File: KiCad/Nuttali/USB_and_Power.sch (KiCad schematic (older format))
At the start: 1 part

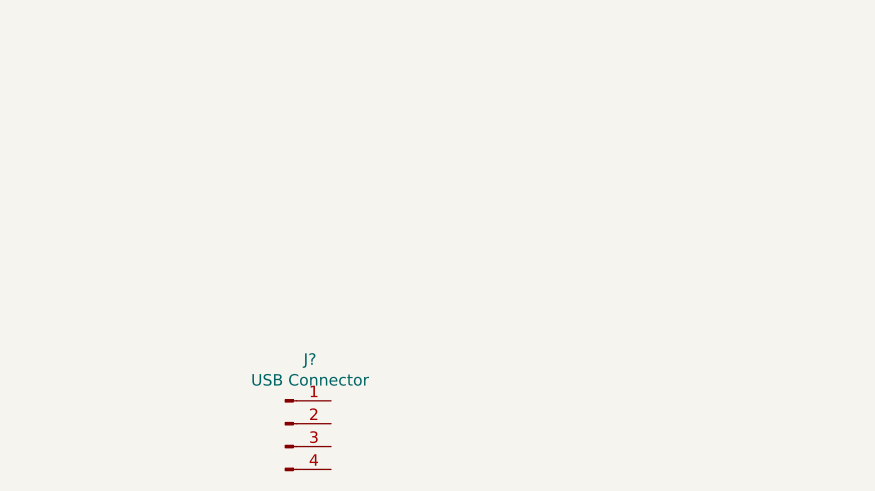
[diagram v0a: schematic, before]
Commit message: Fixed power and USB
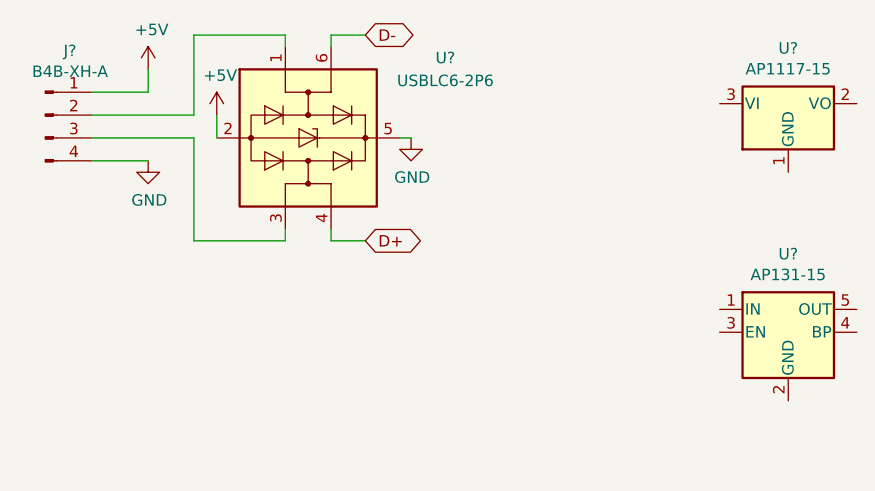
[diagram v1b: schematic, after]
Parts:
- added U?: USBLC6-2P6, Package_TO_SOT_SMD:SOT-666, symbol Power_Protection:USBLC6-2P6
- added U?: AP1117-15, Package_TO_SOT_SMD:SOT-223-3_TabPin2, symbol Regulator_Linear:AP1117-15
- added U?: AP131-15, Package_TO_SOT_SMD:SOT-23-5, symbol Regulator_Linear:AP131-15
- J?: value USB Connector -> B4B-XH-A
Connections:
- net +5V: now reaches J?.1 (Pin_1)
- net +5V: now also U?.2 (GND)
- net at J?.2 (Pin_2): now also U?.1 (I/O1)
- net at J?.3 (Pin_3): now also U?.3 (I/O2)
- net GND: now reaches J?.4 (Pin_4)
- net GND: now also U?.5 (VBUS)
- new net D+: U?.4 (I/O2)
- new net D-: U?.6 (I/O1)
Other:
- moved on the sheet: J?
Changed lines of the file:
@@
 L Connector:Conn_01x04_Male J?
 U 1 1 601D53F8
-P 2450 3050
-F 0 "J?" H 2558 3331 50  0000 C CNN
-F 1 "USB Connector" H 2558 3240 50  0000 C CNN
-F 2 "" H 2450 3050 50  0001 C CNN
-F 3 "~" H 2450 3050 50  0001 C CNN
-	1    2450 3050
+P 1400 1700
+AR Path="/601D53F8" Ref="J?"  Part="1"
+AR Path="/601D470C/601D53F8" Ref="J?"  Part="1"
+F 0 "J?" H 1508 1981 50  0000 C CNN
+F 1 "B4B-XH-A" H 1508 1890 50  0000 C CNN
+F 2 "" H 1400 1700 50  0001 C CNN
+F 3 "~" H 1400 1700 50  0001 C CNN
+	1    1400 1700
 	1    0    0    -1
 $EndComp
+$Comp
+L power:+5V #PWR?
+U 1 1 6025442C
+P 1850 1500
+F 0 "#PWR?" H 1850 1350 50  0001 C CNN
+F 1 "+5V" H 1865 1673 50  0000 C CNN
+F 2 "" H 1850 1500 50  0001 C CNN
+F 3 "" H 1850 1500 50  0001 C CNN
+	1    1850 1500
+	1    0    0    -1
+$EndComp
+Wire Wire Line
+	1600 1600 1850 1600
+Wire Wire Line
+	1850 1600 1850 1500
+$Comp
+L Power_Protection:USBLC6-2P6 U?
+U 1 1 60257671
+P 2550 1800
+F 0 "U?" V 2200 2400 50  0000 C CNN
+F 1 "USBLC6-2P6" V 2300 2400 50  0000 C CNN
+F 2 "Package_TO_SOT_SMD:SOT-666" H 2550 1300 50  0001 C CNN
+F 3 "https://www.st.com/resource/en/datasheet/usblc6-2.pdf" H 2750 2150 50  0001 C CNN
+	1    2550 1800
+	0    1    1    0
+$EndComp
+Wire Wire Line
+	1600 1700 2050 1700
+Wire Wire Line
+	2050 1700 2050 1350
+Wire Wire Line
+	2050 1350 2450 1350
+Wire Wire Line
+	2450 1350 2450 1400
+Wire Wire Line
+	1600 1800 2050 1800
+Wire Wire Line
+	2050 1800 2050 2250
+Wire Wire Line
+	2050 2250 2450 2250
+Wire Wire Line
+	2450 2250 2450 2200
+$Comp
+L power:+5V #PWR?
+U 1 1 60263555
+P 2150 1700
+F 0 "#PWR?" H 2150 1550 50  0001 C CNN
+F 1 "+5V" H 2165 1873 50  0000 C CNN
+F 2 "" H 2150 1700 50  0001 C CNN
+F 3 "" H 2150 1700 50  0001 C CNN
+	1    2150 1700
+	1    0    0    -1
+$EndComp
+Wire Wire Line
+	2150 1800 2150 1700
+Wire Wire Line
+	1600 1900 1850 1900
+$Comp
+L power:GND #PWR?
+U 1 1 60263C21
+P 1850 1900
+F 0 "#PWR?" H 1850 1650 50  0001 C CNN
+F 1 "GND" H 1855 1727 50  0000 C CNN
+F 2 "" H 1850 1900 50  0001 C CNN
+F 3 "" H 1850 1900 50  0001 C CNN
+	1    1850 1900
+	1    0    0    -1
+$EndComp
+Wire Wire Line
+	2950 1800 3000 1800
+$Comp
+L power:GND #PWR?
+U 1 1 6026528C
+P 3000 1800
+F 0 "#PWR?" H 3000 1550 50  0001 C CNN
+F 1 "GND" H 3005 1627 50  0000 C CNN
+F 2 "" H 3000 1800 50  0001 C CNN
+F 3 "" H 3000 1800 50  0001 C CNN
+	1    3000 1800
+	1    0    0    -1
+$EndComp
+Text GLabel 2800 1350 2    50   BiDi ~ 0
+D-
+Text GLabel 2800 2250 2    50   BiDi ~ 0
+D+
+Wire Wire Line
+	2800 1350 2650 1350
+Wire Wire Line
+	2650 1350 2650 1400
+Wire Wire Line
+	2800 2250 2650 2250
+Wire Wire Line
+	2650 2250 2650 2200
+$Comp
+L Regulator_Linear:AP1117-15 U?
+U 1 1 60275CC9
+P 4650 1650
+F 0 "U?" H 4650 1892 50  0000 C CNN
+F 1 "AP1117-15" H 4650 1801 50  0000 C CNN
+F 2 "Package_TO_SOT_SMD:SOT-223-3_TabPin2" H 4650 1850 50  0001 C CNN
+F 3 "http://www.diodes.com/datasheets/AP1117.pdf" H 4750 1400 50  0001 C CNN
+	1    4650 1650
+	1    0    0    -1
+$EndComp
+$Comp
+L Regulator_Linear:AP131-15 U?
+U 1 1 602779E7
+P 4650 2650
+F 0 "U?" H 4650 2992 50  0000 C CNN
+F 1 "AP131-15" H 4650 2901 50  0000 C CNN
+F 2 "Package_TO_SOT_SMD:SOT-23-5" H 4650 2975 50  0001 C CNN
+F 3 "http://www.diodes.com/_files/datasheets/AP131.pdf" H 4650 2650 50  0001 C CNN
+	1    4650 2650
+	1    0    0    -1
+$EndComp
